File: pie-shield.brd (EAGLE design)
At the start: 35.1 x 37.2 mm, 20 parts, among them IC4 NRF24L01SMD, Q2 3.2X2.5CRYSTAL

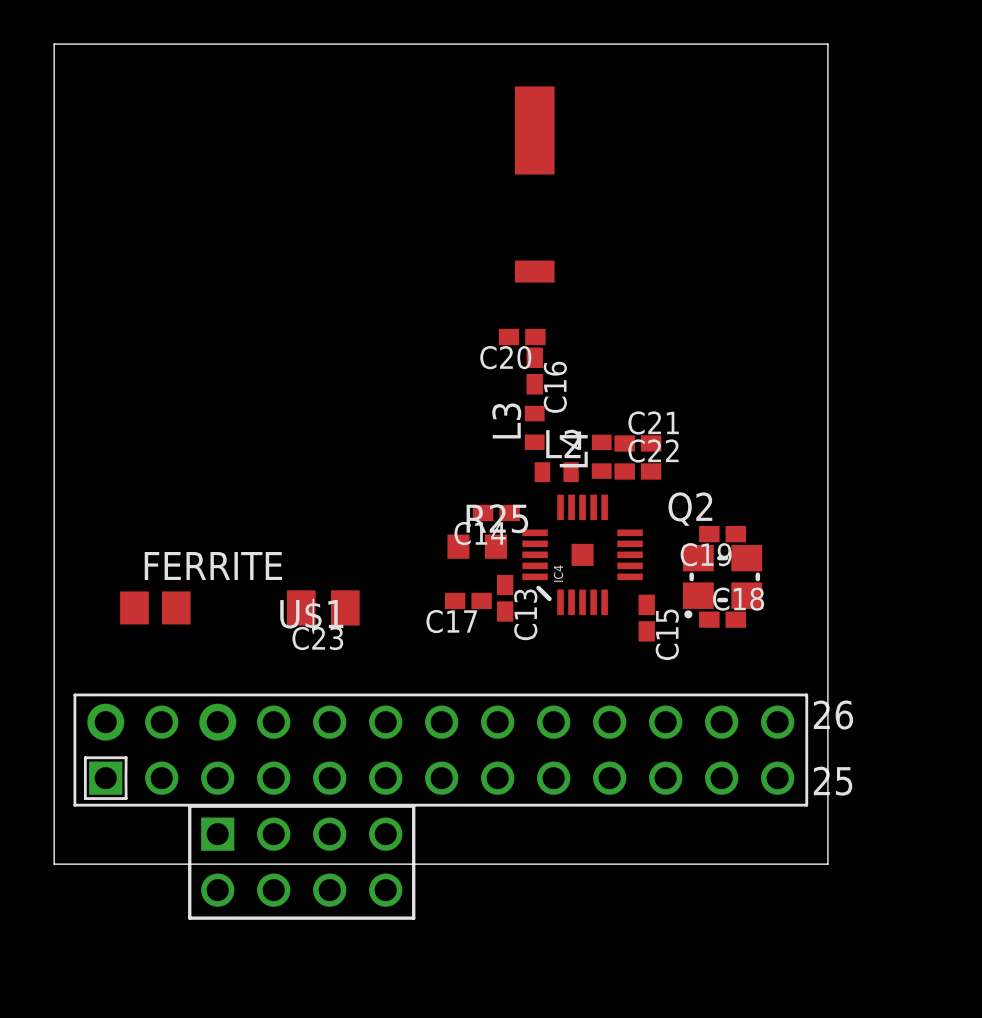
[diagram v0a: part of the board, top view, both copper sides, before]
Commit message: minisized
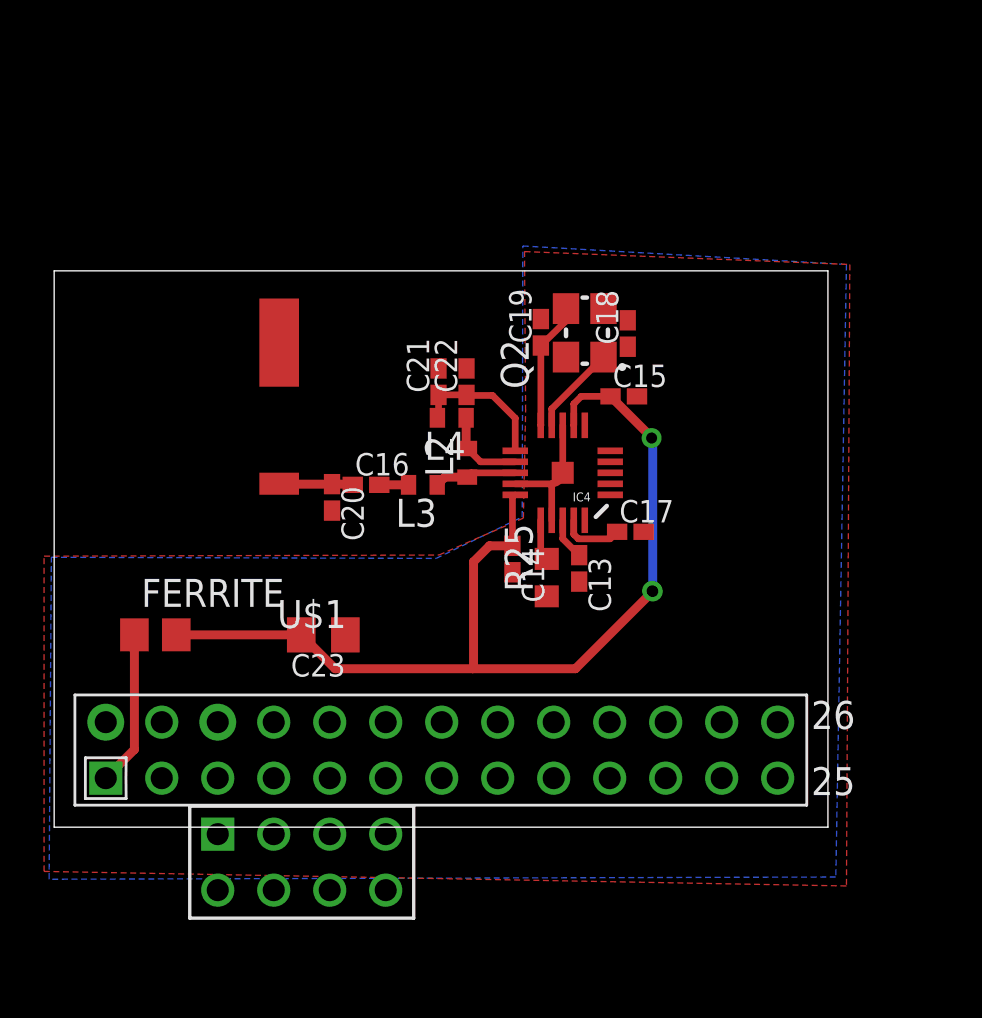
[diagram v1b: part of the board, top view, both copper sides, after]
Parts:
- moved ANT 15.1 mm to (10.2, 19.7)
- moved C18 13.7 mm to (26.0, 24.1), turned to 90 degrees
- moved Q2 12.7 mm to (24.1, 24.1), turned to 90 degrees
- moved C19 12.3 mm to (22.1, 24.1), turned to 90 degrees
- moved C20 11.3 mm to (12.6, 16.6), turned to 270 degrees
- moved C15 10.1 mm to (25.8, 21.2), turned to 0 degrees
- moved C21 9.47 mm to (17.4, 21.9), turned to 90 degrees
- moved C16 9.23 mm to (14.1, 17.2), turned to 0 degrees
- moved C22 8.78 mm to (18.7, 21.9), turned to 90 degrees
- moved C17 7.99 mm to (26.1, 15.1), turned to 0 degrees
- moved L4 7.03 mm to (18.0, 20.2), turned to 180 degrees
- moved L3 5.69 mm to (16.7, 17.2), turned to 180 degrees
- moved L2 4.09 mm to (18.7, 18.2), turned to 90 degrees
- moved IC4 3.83 mm to (23.1, 17.8), turned to 180 degrees
- moved C13 3.62 mm to (23.8, 13.4)
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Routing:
- net +3V3_RF: track 0.00 -> 47.4 mm, vias 0 -> 3
- net +3V3: track 0.00 -> 7.04 mm
- net N$73: track 0.00 -> 6.46 mm
- net GND: track 0.00 -> 6.17 mm
- net N$11: track 0.00 -> 5.78 mm
- net N$10: track 0.00 -> 4.07 mm
- net N$78: track 0.00 -> 3.84 mm
- net N$79: track 0.00 -> 3.77 mm
- net N$12: track 0.00 -> 3.36 mm
- net N$70: track 0.00 -> 2.82 mm
- net N$71: track 0.00 -> 1.86 mm
- net N$80: track 0.00 -> 1.33 mm
- added copper zone on layer 1, net GND
- added copper zone on layer 16, net GND
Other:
- board size 35.1 x 37.2 mm -> 35.1 x 25.2 mm
